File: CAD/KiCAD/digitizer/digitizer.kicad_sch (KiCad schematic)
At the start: 1 part, among them J1 Conn_01x06

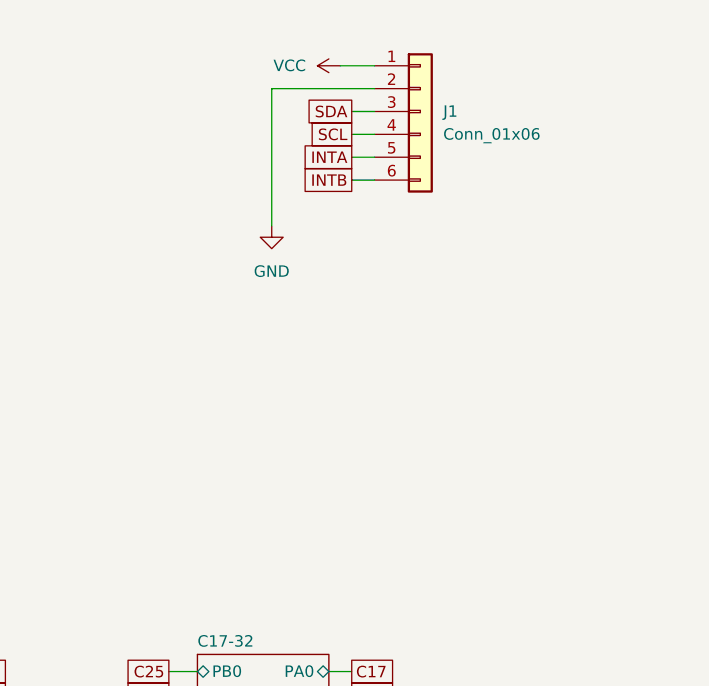
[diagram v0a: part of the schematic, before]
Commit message: wip
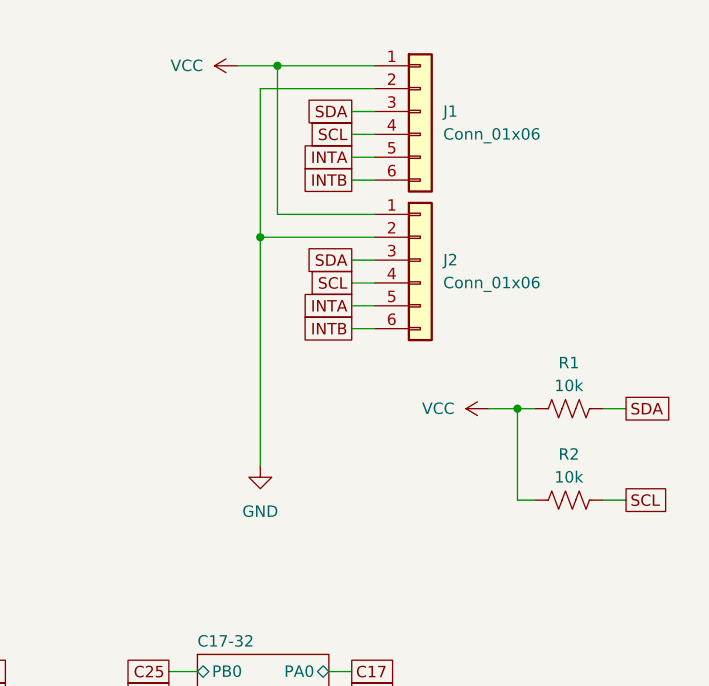
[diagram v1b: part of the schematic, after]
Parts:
- added J2: Conn_01x06, Connector_PinHeader_2.54mm:PinHeader_1x06_P2.54mm_Vertical, symbol Connector_Generic:Conn_01x06
- added R1, R2: 10k, Resistor_THT:R_Axial_DIN0207_L6.3mm_D2.5mm_P15.24mm_Horizontal, symbol Device:R_US
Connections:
- net GND: now also J2.2 (Pin_2)
- net INTA: now also J2.5 (Pin_5)
- net INTB: now also J2.6 (Pin_6)
- net SCL: now also J2.4 (Pin_4), R2.2
- net SDA: now also J2.3 (Pin_3), R1.2
- net VCC: now also J2.1 (Pin_1), R1.1, R2.1
